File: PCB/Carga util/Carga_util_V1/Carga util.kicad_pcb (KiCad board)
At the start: 2 copper layers, 48.5 x 50 mm, 30 parts, among them J1 CONN, J2 BG51, J3 DEBUG, SW1 Reset, U1 ATtiny85-20S, U2 LM1117DT-3.3

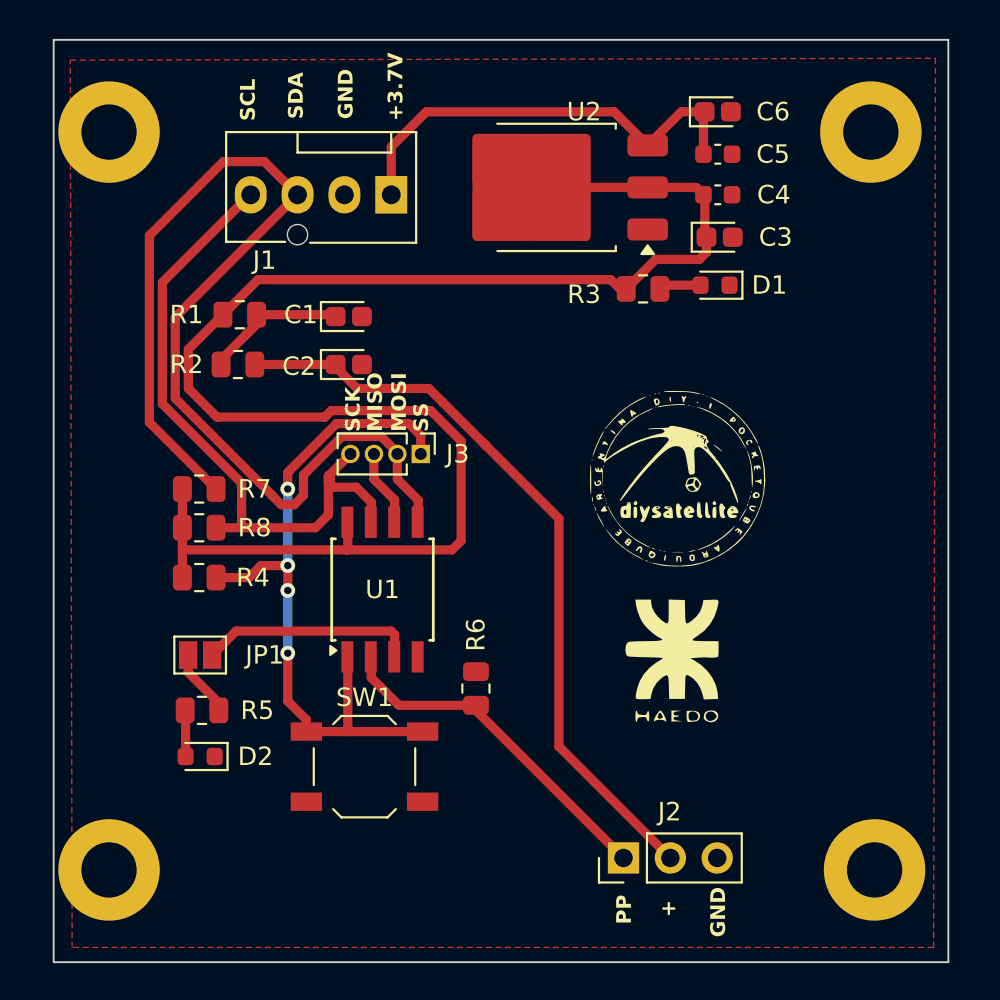
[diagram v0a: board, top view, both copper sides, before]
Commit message: nuevo pcb
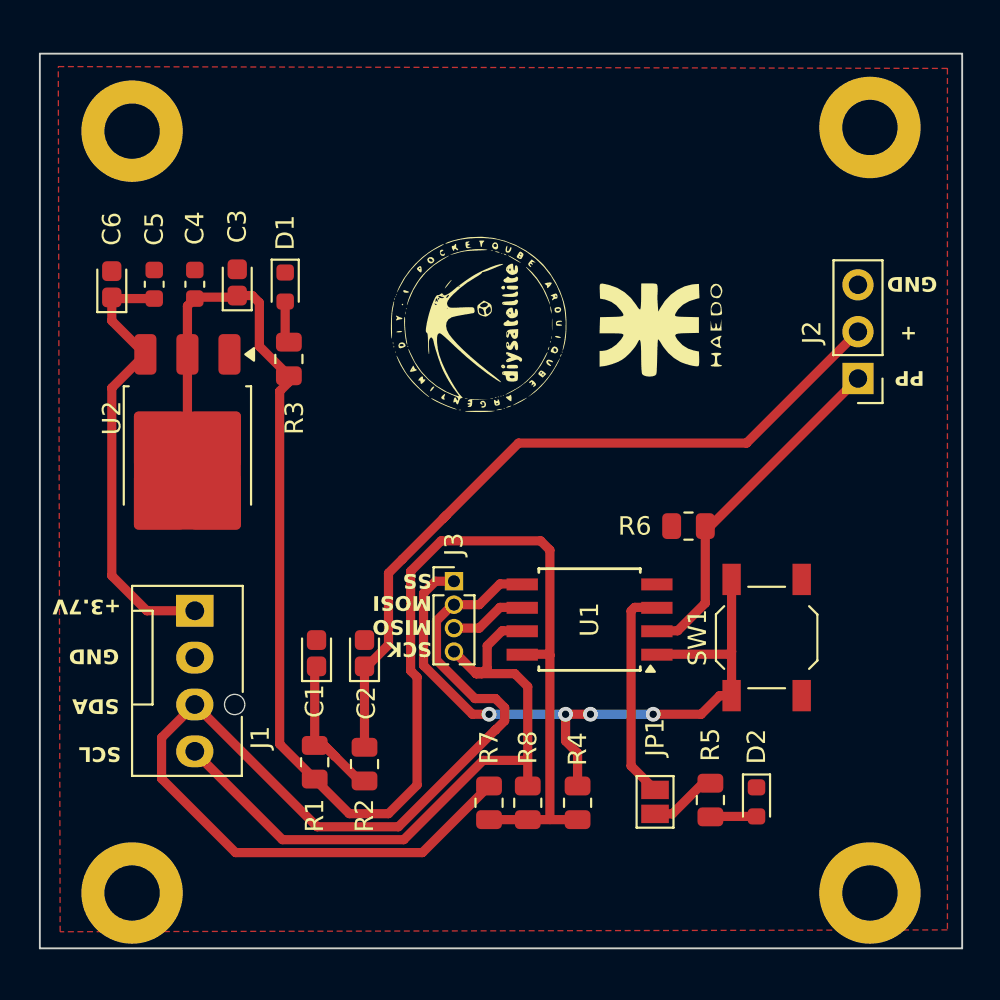
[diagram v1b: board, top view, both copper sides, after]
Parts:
- moved G*** 53.6 mm to (153.5, 63.0), turned to 90 degrees
- moved ? 41.3 mm to (167.2, 121.6), turned to 90 degrees
- moved REF** 41.3 mm to (127.2, 121.6), turned to 90 degrees
- moved ? 40.3 mm to (167.2, 80.1), turned to 90 degrees
- moved ? 40.1 mm to (127.2, 80.3), turned to 90 degrees
- moved C6 34.2 mm to (126.1, 88.6), turned to 90 degrees
- moved C5 31.4 mm to (128.4, 88.6), turned to 90 degrees
- moved D2 30.3 mm to (161.0, 116.7), turned to -90 degrees
- moved J2 28.9 mm to (166.5, 93.7), turned to 180 degrees
- moved C4 28.8 mm to (130.6, 88.6), turned to 90 degrees
- moved R5 28.0 mm to (158.5, 116.6), turned to -90 degrees
- moved C3 26.3 mm to (132.9, 88.5), turned to 90 degrees
- moved JP1 25.9 mm to (155.5, 116.7), turned to 90 degrees
- moved J1 24.9 mm to (130.6, 106.3), turned to -90 degrees
- moved R1 24.6 mm to (137.1, 114.5), turned to 90 degrees
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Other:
- board size 48.5 x 50 mm -> 50 x 48.5 mm
